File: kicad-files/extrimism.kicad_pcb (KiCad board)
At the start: 2 copper layers, 77 x 46 mm, 31 parts, among them SW1 SW_Push, SW10 SW_Push, SW11 SW_Push, SW12 SW_Push, SW2 SW_Push, SW3 SW_Push, SW4 SW_Push, SW5 SW_Push, SW6 SW_Push, SW7 SW_Push, SW8 SW_Push, SW9 SW_Push, U1 Pico, U2 RFM95W-868S2

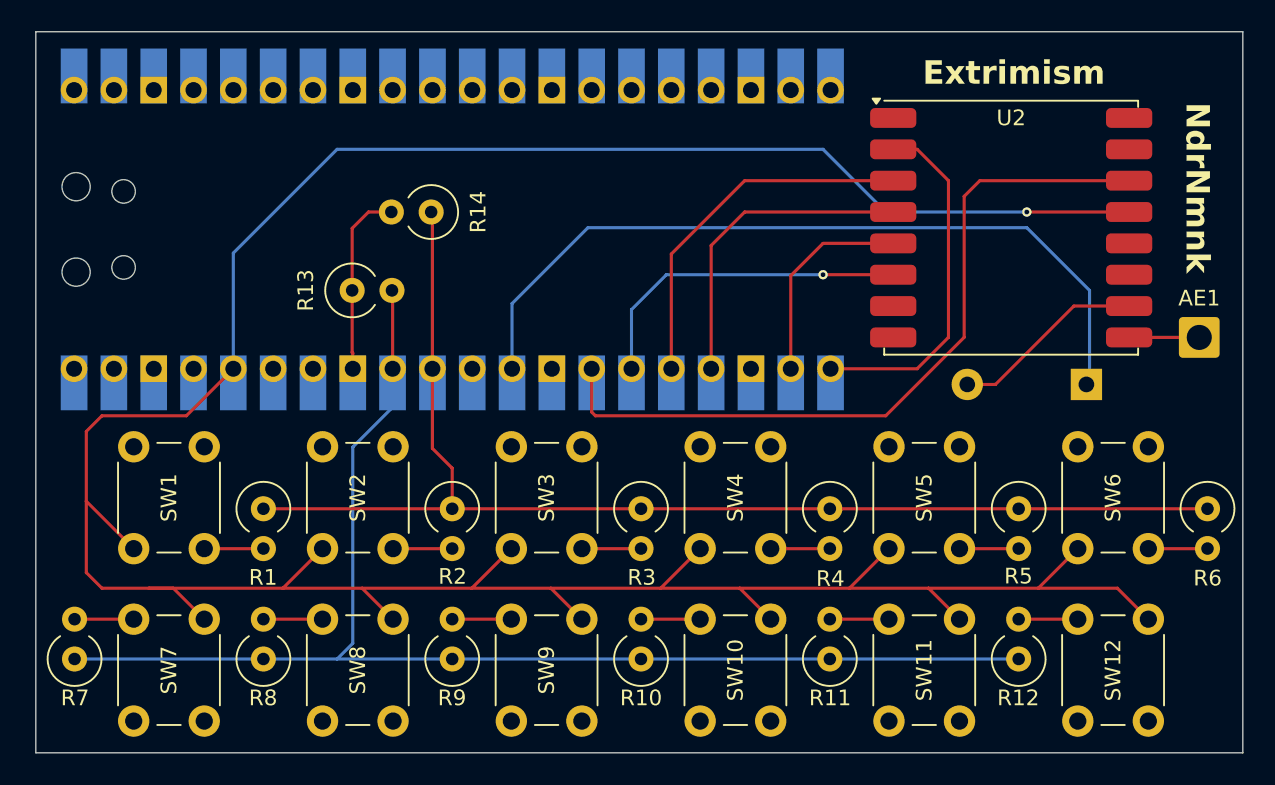
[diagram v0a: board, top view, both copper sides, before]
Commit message: updated PCB design
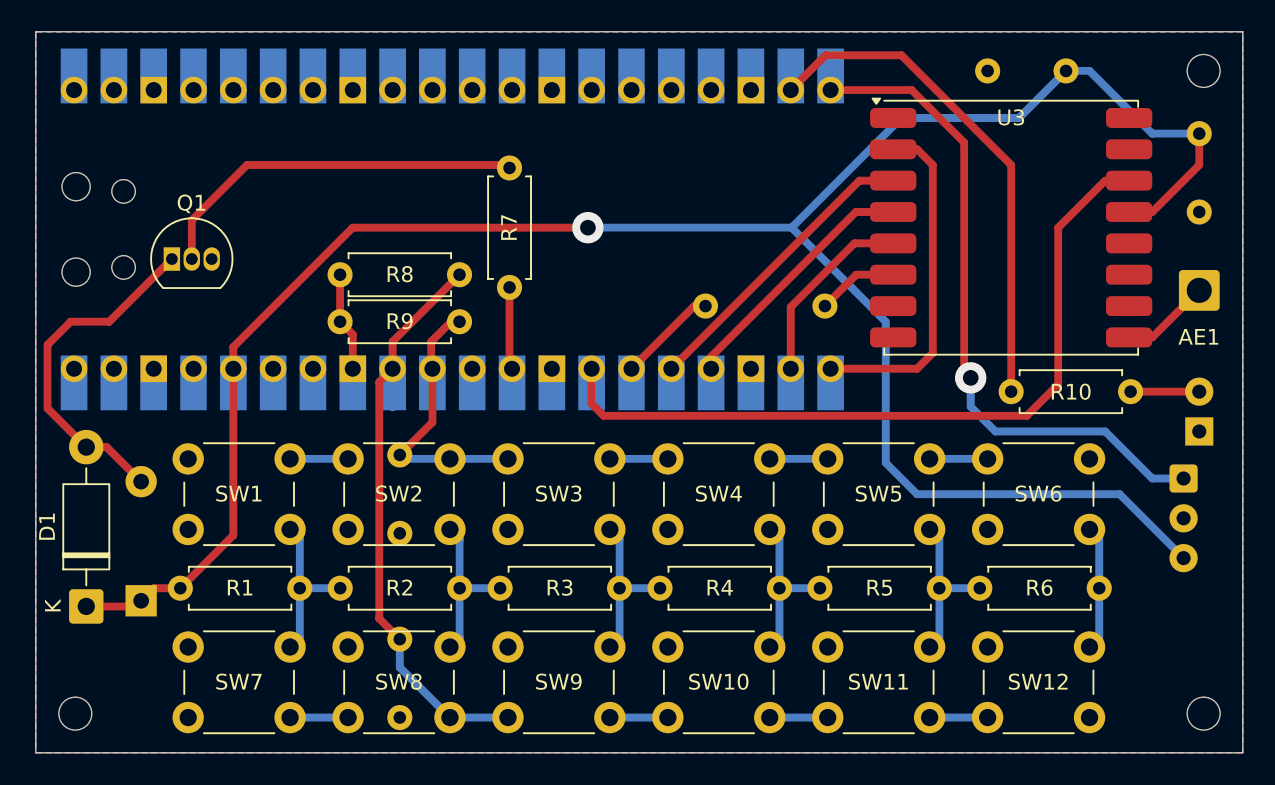
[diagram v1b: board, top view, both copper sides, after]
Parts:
- removed R12: 15k, Resistor_THT:R_Axial_DIN0309_L9.0mm_D3.2mm_P2.54mm_Vertical
- removed the R8 at (54.3, 115.5)
- removed the R9 at (66.3, 115.5)
- added C1: 10nF, Capacitor_THT:C_Disc_D5.0mm_W2.5mm_P5.00mm, B.Cu at (63.0, 102.5)
- added C2: 10nF, Capacitor_THT:C_Disc_D5.0mm_W2.5mm_P5.00mm, B.Cu at (63.0, 114.2)
- added C3: 100uF, Capacitor_THT:C_Disc_D5.0mm_W2.5mm_P5.00mm, B.Cu at (105.5, 78.0)
- added C4: 100nF, Capacitor_THT:C_Disc_D5.0mm_W2.5mm_P5.00mm, B.Cu at (114.0, 82.0)
- added D1: 1N4001, Diode_THT:D_DO-41_SOD81_P10.16mm_Horizontal, F.Cu at (43.0, 112.2)
- added D2: IR_LED, LED_THT:LED_D3.0mm, B.Cu at (114.0, 101.0)
- added H1: MountingHole, MountingHole:MountingHole_2.1mm, F.Cu at (114.3, 78.0)
- added H2: MountingHole, MountingHole:MountingHole_2.1mm, F.Cu at (114.3, 119.0)
- added H3: MountingHole, MountingHole:MountingHole_2.1mm, F.Cu at (42.3, 119.0)
- added Q1: NPN, Package_TO_SOT_THT:TO-92_Inline, F.Cu at (48.5, 90.0)
- added U1: TSOP38238, OptoDevice:Vishay_MINICAST-3Pin, B.Cu at (113.0, 104.0)
- R1, R7: footprint Resistor_THT:R_Axial_DIN0309_L9.0mm_D3.2mm_P2.54mm_Vertical -> Resistor_THT:R_Axial_DIN0207_L6.3mm_D2.5mm_P7.62mm_Horizontal
- R10: value 6.8k -> 470; footprint Resistor_THT:R_Axial_DIN0309_L9.0mm_D3.2mm_P2.54mm_Vertical -> Resistor_THT:R_Axial_DIN0207_L6.3mm_D2.5mm_P7.62mm_Horizontal
- R11: value 10k -> 0; footprint Resistor_THT:R_Axial_DIN0309_L9.0mm_D3.2mm_P2.54mm_Vertical -> Resistor_THT:R_Axial_DIN0207_L6.3mm_D2.5mm_P7.62mm_Horizontal; moved to B.Cu
- R2: value 2.2k -> 1.2k; footprint Resistor_THT:R_Axial_DIN0309_L9.0mm_D3.2mm_P2.54mm_Vertical -> Resistor_THT:R_Axial_DIN0207_L6.3mm_D2.5mm_P7.62mm_Horizontal
- R3: value 4k -> 1.8k; footprint Resistor_THT:R_Axial_DIN0309_L9.0mm_D3.2mm_P2.54mm_Vertical -> Resistor_THT:R_Axial_DIN0207_L6.3mm_D2.5mm_P7.62mm_Horizontal
- R4: value 6.8k -> 2.7k; footprint Resistor_THT:R_Axial_DIN0309_L9.0mm_D3.2mm_P2.54mm_Vertical -> Resistor_THT:R_Axial_DIN0207_L6.3mm_D2.5mm_P7.62mm_Horizontal
- R5: value 10k -> 3.3k; footprint Resistor_THT:R_Axial_DIN0309_L9.0mm_D3.2mm_P2.54mm_Vertical -> Resistor_THT:R_Axial_DIN0207_L6.3mm_D2.5mm_P7.62mm_Horizontal
- R6: value 15k -> 4.7k; footprint Resistor_THT:R_Axial_DIN0309_L9.0mm_D3.2mm_P2.54mm_Vertical -> Resistor_THT:R_Axial_DIN0207_L6.3mm_D2.5mm_P7.62mm_Horizontal
- R8: renamed from R13; footprint Resistor_THT:R_Axial_DIN0309_L9.0mm_D3.2mm_P2.54mm_Vertical -> Resistor_THT:R_Axial_DIN0207_L6.3mm_D2.5mm_P7.62mm_Horizontal
- R9: renamed from R14; footprint Resistor_THT:R_Axial_DIN0309_L9.0mm_D3.2mm_P2.54mm_Vertical -> Resistor_THT:R_Axial_DIN0207_L6.3mm_D2.5mm_P7.62mm_Horizontal
- moved BZ1 61.9 mm to (46.5, 111.8), turned to 90 degrees
- moved R7 36.5 mm to (70.0, 91.8)
- moved R10 29.1 mm to (102.0, 98.5), turned to 0 degrees
- moved R11 23.9 mm to (82.5, 93.0), turned to 0 degrees
- moved R6 15.4 mm to (100.0, 111.0), turned to 0 degrees
- moved R5 13.7 mm to (89.8, 111.0), turned to 0 degrees
- moved R4 12.0 mm to (79.6, 111.0), turned to 0 degrees
- moved SW12 10.4 mm to (100.5, 114.8), turned to 0 degrees
- moved R3 10.3 mm to (69.4, 111.0), turned to 0 degrees
- moved R2 8.76 mm to (59.2, 111.0), turned to 0 degrees
- moved SW11 8.59 mm to (90.3, 114.8), turned to 0 degrees
- moved SW6 8.12 mm to (100.5, 102.8), turned to 0 degrees
- moved R1 7.33 mm to (49.0, 111.0), turned to 0 degrees
- moved R9 7.23 mm to (66.8, 94.0)
- moved SW5 6.93 mm to (90.3, 102.8), turned to 0 degrees
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- renumbered U1 to U2, U2 to U3
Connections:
- BZ1 pad 1: /buzz -> /3v3
- BZ1 pad 2: GND -> Net-(BZ1--)
- R1 pad 1: /adc0 -> /3v3
- R10 pad 1: /adc1 -> /ir_tx
- R10 pad 2: Net-(R10-Pad2) -> Net-(D2-A)
- R11 pad 1: /adc1 -> Net-(U2-GPIO20)
- R11 pad 2: Net-(R11-Pad2) -> Net-(U3-RESET)
- R2 pad 1: /adc0 -> Net-(R1-Pad2)
- R3 pad 1: /adc0 -> Net-(R2-Pad2)
- R4 pad 1: /adc0 -> Net-(R3-Pad2)
- R5 pad 1: /adc0 -> Net-(R4-Pad2)
- R6 pad 1: /adc0 -> Net-(R5-Pad2)
- R7 pad 1: /adc1 -> /buzz
- R7 pad 2: Net-(R7-Pad2) -> Net-(Q1-B)
- SW1 pad 1: /3v3_kb -> /adc0
- SW10 pad 1: /3v3_kb -> Net-(R4-Pad2)
- SW10 pad 2: Net-(R10-Pad2) -> /adc1
- SW11 pad 1: /3v3_kb -> Net-(R5-Pad2)
- SW11 pad 2: Net-(R11-Pad2) -> /adc1
- SW12 pad 1: /3v3_kb -> Net-(R6-Pad2)
- SW12 pad 2: Net-(R12-Pad2) -> /adc1
- SW2 pad 1: /3v3_kb -> /adc0
- SW3 pad 1: /3v3_kb -> /adc0
- SW4 pad 1: /3v3_kb -> /adc0
- SW5 pad 1: /3v3_kb -> /adc0
- SW6 pad 1: /3v3_kb -> /adc0
- SW7 pad 1: /3v3_kb -> Net-(R1-Pad2)
- SW7 pad 2: Net-(R7-Pad2) -> /adc1
- SW8 pad 1: /3v3_kb -> Net-(R2-Pad2)
- SW8 pad 2: Net-(R8-Pad2) -> /adc1
- SW9 pad 1: /3v3_kb -> Net-(R3-Pad2)
- SW9 pad 2: Net-(R9-Pad2) -> /adc1
- U2 pad 18: unconnected-(U1-GND-Pad18)_1 -> GND
- U2 pad 19: unconnected-(U1-GPIO14-Pad19) -> /ir_tx
- U2 pad 20: unconnected-(U1-GPIO15-Pad20) -> /ir_rx
- U2 pad 23: unconnected-(U1-GND-Pad23) -> GND
- U2 pad 26: Net-(U1-GPIO20) -> Net-(U2-GPIO20)
- U2 pad 28: unconnected-(U1-GND-Pad28) -> GND
- U2 pad 36: /3v3_kb -> /3v3
- U2 pad 38: Net-(BC1-load-) -> GND
- U3 pad 1: unconnected-(U2-GND-Pad1) -> GND
- U3 pad 13: /3v3_kb -> /3v3
- U3 pad 6: Net-(U1-GPIO20) -> Net-(U3-RESET)
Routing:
- net /3v3_kb: track 197.2 -> 0.00 mm, vias 1 -> 0
- net /3v3: track 0.00 -> 140.6 mm, vias 0 -> 1
- net /adc0: track 80.1 -> 32.9 mm
- net /buzz: track 50.7 -> 5.48 mm
- net /ir_rx: track 0.00 -> 42.4 mm, vias 0 -> 1
- net /ir_tx: track 0.00 -> 32.3 mm
- net /adc1: track 85.2 -> 54.2 mm
- net Net-(Q1-B): track 0.00 -> 24.5 mm
- net Net-(BZ1--): track 0.00 -> 22.2 mm
- net Net-(U1-GPIO20): track 21.4 -> 0.00 mm, vias 1 -> 0
- net GND: track 12.4 -> 1.13 mm
- net Net-(R4-Pad2): track 3.77 -> 10.6 mm
- net Net-(R2-Pad2): track 3.77 -> 10.6 mm
- net Net-(R5-Pad2): track 3.77 -> 10.6 mm
- net Net-(R1-Pad2): track 3.77 -> 10.6 mm
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- added copper zone on B.Cu, net GND
- added copper zone on F.Cu, net GND
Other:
- board text added: "X3mist"
- board text removed: "Extrimism"
- board text removed: "SW11"
